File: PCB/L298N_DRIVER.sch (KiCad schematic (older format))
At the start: 21 parts, among them J1 PWM-INPUT, J2 MOT-OUTPUT, J3 +5V, J4 +BATT, J5 SERIAL, J6 I2C, U1 L298N, U2 adino2

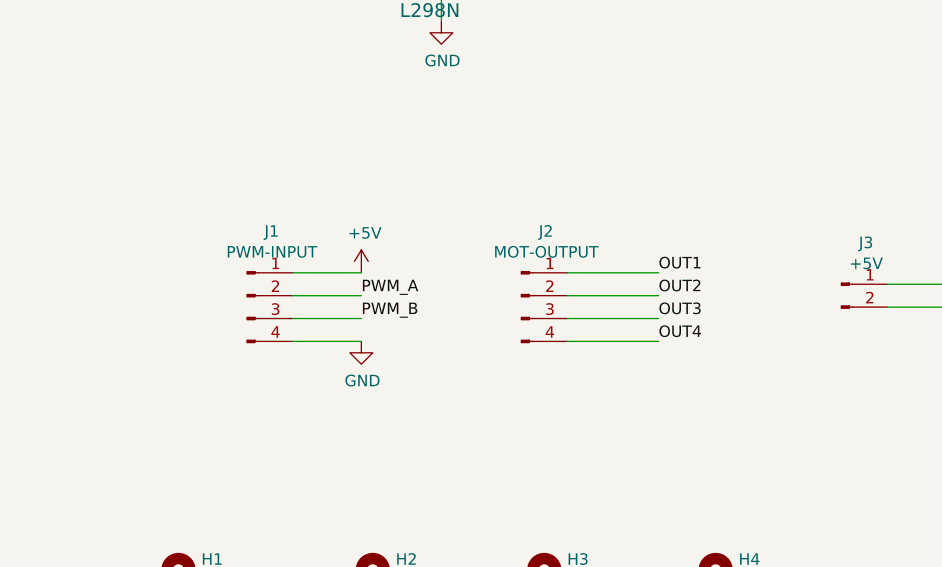
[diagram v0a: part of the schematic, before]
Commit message: pcb update
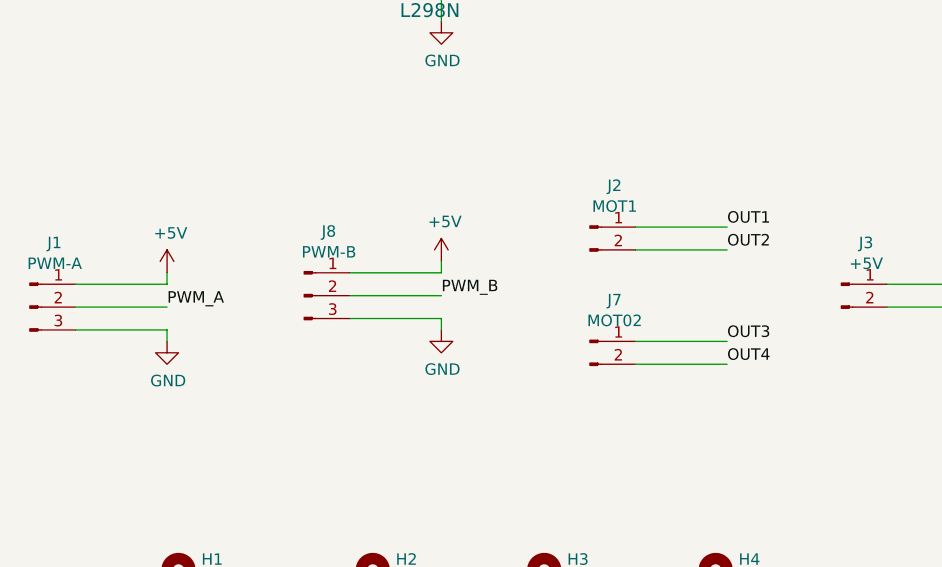
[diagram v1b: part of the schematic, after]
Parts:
- removed J1: PWM-INPUT, Connector_JST:JST_PH_S4B-PH-K_1x04_P2.00mm_Horizontal, symbol Connector:Conn_01x04_Male
- removed J2: MOT-OUTPUT, Connector_JST:JST_PH_S4B-PH-K_1x04_P2.00mm_Horizontal, symbol Connector:Conn_01x04_Male
- added J1: PWM-A, Connector_JST:JST_PH_S3B-PH-K_1x03_P2.00mm_Horizontal, symbol Connector:Conn_01x03_Male
- added J2: MOT1, Connector_JST:JST_PH_S2B-PH-K_1x02_P2.00mm_Horizontal, symbol Connector:Conn_01x02_Male
- added J7: MOT02, Connector_JST:JST_PH_S2B-PH-K_1x02_P2.00mm_Horizontal, symbol Connector:Conn_01x02_Male
- added J8: PWM-B, Connector_JST:JST_PH_S3B-PH-K_1x03_P2.00mm_Horizontal, symbol Connector:Conn_01x03_Male
- J5, J6: footprint Connector_JST:JST_PH_S4B-PH-K_1x04_P2.00mm_Horizontal -> Connector_JST:JST_PH_B4B-PH-K_1x04_P2.00mm_Vertical
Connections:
- net +5V: now also J1.1 (Pin_1), J8.1 (Pin_1)
- net GND: now also J1.3 (Pin_3), J8.3 (Pin_3)
- net OUT1: now also J2.1 (Pin_1)
- net OUT2: now also J2.2 (Pin_2)
- net OUT3: now also J7.1 (Pin_1)
- net OUT4: now also J7.2 (Pin_2)
- net PWM_A: now also J1.2 (Pin_2)
- net PWM_B: now also J8.2 (Pin_2)
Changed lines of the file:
@@
 Wire Wire Line
 	8200 3150 8600 3150
-Wire Wire Line
-	2650 5700 2950 5700
 $Comp
 L power:GND #PWR04
 U 1 1 5E721439
-P 2950 5700
-F 0 "#PWR04" H 2950 5450 50  0001 C CNN
-F 1 "GND" H 2955 5527 50  0000 C CNN
-F 2 "" H 2950 5700 50  0001 C CNN
-F 3 "" H 2950 5700 50  0001 C CNN
-	1    2950 5700
+P 2100 5700
+F 0 "#PWR04" H 2100 5450 50  0001 C CNN
+F 1 "GND" H 2105 5527 50  0000 C CNN
+F 2 "" H 2100 5700 50  0001 C CNN
+F 3 "" H 2100 5700 50  0001 C CNN
+	1    2100 5700
 	1    0    0    -1
 $EndComp
@@
 Text Label 8600 3150 0    50   ~ 0
 PWM_B
-Text Label 2950 5500 0    50   ~ 0
+Text Label 2100 5550 0    50   ~ 0
 PWM_A
-Text Label 2950 5600 0    50   ~ 0
-PWM_B
 $Comp
 L power:GND #PWR013
@@
 $EndComp
 $Comp
-L Connector:Conn_01x04_Male J1
-U 1 1 5E80A4BE
-P 2450 5500
-F 0 "J1" H 2558 5781 50  0000 C CNN
-F 1 "PWM-INPUT" H 2558 5690 50  0000 C CNN
-F 2 "Connector_JST:JST_PH_S4B-PH-K_1x04_P2.00mm_Horizontal" H 2450 5500 50  0001 C CNN
-F 3 "~" H 2450 5500 50  0001 C CNN
-	1    2450 5500
-	1    0    0    -1
-$EndComp
-Wire Wire Line
-	2650 5500 2950 5500
-Wire Wire Line
-	2650 5600 2950 5600
-$Comp
 L power:+5V #PWR06
 U 1 1 5E80EB83
-P 2950 5400
-F 0 "#PWR06" H 2950 5250 50  0001 C CNN
-F 1 "+5V" H 2965 5573 50  0000 C CNN
-F 2 "" H 2950 5400 50  0001 C CNN
-F 3 "" H 2950 5400 50  0001 C CNN
-	1    2950 5400
-	1    0    0    -1
-$EndComp
-$Comp
-L Connector:Conn_01x04_Male J2
-U 1 1 5E81BECC
-P 3650 5500
-F 0 "J2" H 3758 5781 50  0000 C CNN
-F 1 "MOT-OUTPUT" H 3758 5690 50  0000 C CNN
-F 2 "Connector_JST:JST_PH_S4B-PH-K_1x04_P2.00mm_Horizontal" H 3650 5500 50  0001 C CNN
-F 3 "~" H 3650 5500 50  0001 C CNN
-	1    3650 5500
-	1    0    0    -1
-$EndComp
-Text Label 4250 5400 0    50   ~ 0
+P 2100 5400
+F 0 "#PWR06" H 2100 5250 50  0001 C CNN
+F 1 "+5V" H 2115 5573 50  0000 C CNN
+F 2 "" H 2100 5400 50  0001 C CNN
+F 3 "" H 2100 5400 50  0001 C CNN
+	1    2100 5400
+	1    0    0    -1
+$EndComp
+Text Label 4550 5200 0    50   ~ 0
 OUT1
-Text Label 4250 5500 0    50   ~ 0
+Text Label 4550 5300 0    50   ~ 0
 OUT2
 Wire Wire Line
-	3850 5700 4250 5700
-Text Label 4250 5700 0    50   ~ 0
+	4150 5800 4550 5800
+Text Label 4550 5800 0    50   ~ 0
 OUT4
-Text Label 4250 5600 0    50   ~ 0
+Text Label 4550 5700 0    50   ~ 0
 OUT3
 Wire Wire Line
-	3850 5600 4250 5600
-Wire Wire Line
-	3850 5400 4250 5400
-Wire Wire Line
-	3850 5500 4250 5500
+	4150 5700 4550 5700
+Wire Wire Line
+	4150 5200 4550 5200
+Wire Wire Line
+	4150 5300 4550 5300
 $Comp
 L Connector:Conn_01x04_Male J5
@@
 F 0 "J5" H 7508 5731 50  0000 C CNN
 F 1 "SERIAL" H 7508 5640 50  0000 C CNN
-F 2 "Connector_JST:JST_PH_S4B-PH-K_1x04_P2.00mm_Horizontal" H 7400 5450 50  0001 C CNN
+F 2 "Connector_JST:JST_PH_B4B-PH-K_1x04_P2.00mm_Vertical" H 7400 5450 50  0001 C CNN
 F 3 "~" H 7400 5450 50  0001 C CNN
 	1    7400 5450
@@
 F 0 "J6" H 8908 5731 50  0000 C CNN
 F 1 "I2C" H 8908 5640 50  0000 C CNN
-F 2 "Connector_JST:JST_PH_S4B-PH-K_1x04_P2.00mm_Horizontal" H 8800 5450 50  0001 C CNN
+F 2 "Connector_JST:JST_PH_B4B-PH-K_1x04_P2.00mm_Vertical" H 8800 5450 50  0001 C CNN
 F 3 "~" H 8800 5450 50  0001 C CNN
 	1    8800 5450
@@
 Text Label 9650 5550 0    50   ~ 0
 SDA
-Wire Wire Line
-	2650 5400 2950 5400
+$Comp
+L Connector:Conn_01x02_Male J2
+U 1 1 5E811B91
+P 3950 5200
+F 0 "J2" H 4058 5381 50  0000 C CNN
+F 1 "MOT1" H 4058 5290 50  0000 C CNN
+F 2 "Connector_JST:JST_PH_S2B-PH-K_1x02_P2.00mm_Horizontal" H 3950 5200 50  0001 C CNN
+F 3 "~" H 3950 5200 50  0001 C CNN
+	1    3950 5200
+	1    0    0    -1
+$EndComp
+$Comp
+L Connector:Conn_01x02_Male J7
+U 1 1 5E8159E2
+P 3950 5700
+F 0 "J7" H 4058 5881 50  0000 C CNN
+F 1 "MOT02" H 4058 5790 50  0000 C CNN
+F 2 "Connector_JST:JST_PH_S2B-PH-K_1x02_P2.00mm_Horizontal" H 3950 5700 50  0001 C CNN
+F 3 "~" H 3950 5700 50  0001 C CNN
+	1    3950 5700
+	1    0    0    -1
+$EndComp
+$Comp
+L Connector:Conn_01x03_Male J1
+U 1 1 5E8405FC
+P 1500 5550
+F 0 "J1" H 1608 5831 50  0000 C CNN
+F 1 "PWM-A" H 1608 5740 50  0000 C CNN
+F 2 "Connector_JST:JST_PH_S3B-PH-K_1x03_P2.00mm_Horizontal" H 1500 5550 50  0001 C CNN
+F 3 "~" H 1500 5550 50  0001 C CNN
+	1    1500 5550
+	1    0    0    -1
+$EndComp
+$Comp
+L power:GND #PWR020
+U 1 1 5E84B54A
+P 3300 5650
+F 0 "#PWR020" H 3300 5400 50  0001 C CNN
+F 1 "GND" H 3305 5477 50  0000 C CNN
+F 2 "" H 3300 5650 50  0001 C CNN
+F 3 "" H 3300 5650 50  0001 C CNN
+	1    3300 5650
+	1    0    0    -1
+$EndComp
+$Comp
+L power:+5V #PWR019
+U 1 1 5E84B551
+P 3300 5350
+F 0 "#PWR019" H 3300 5200 50  0001 C CNN
+F 1 "+5V" H 3315 5523 50  0000 C CNN
+F 2 "" H 3300 5350 50  0001 C CNN
+F 3 "" H 3300 5350 50  0001 C CNN
+	1    3300 5350
+	1    0    0    -1
+$EndComp
+Wire Wire Line
+	1700 5450 2100 5450
+Wire Wire Line
+	2100 5450 2100 5400
+Wire Wire Line
+	1700 5550 2100 5550
+Wire Wire Line
+	1700 5650 2100 5650
+Wire Wire Line
+	2100 5650 2100 5700
+Wire Wire Line
+	3300 5400 3300 5350
+Text Label 3300 5500 0    50   ~ 0
+PWM_B
+$Comp
+L Connector:Conn_01x03_Male J8
+U 1 1 5E84B557
+P 2700 5500
+F 0 "J8" H 2808 5781 50  0000 C CNN
+F 1 "PWM-B" H 2808 5690 50  0000 C CNN
+F 2 "Connector_JST:JST_PH_S3B-PH-K_1x03_P2.00mm_Horizontal" H 2700 5500 50  0001 C CNN
+F 3 "~" H 2700 5500 50  0001 C CNN
+	1    2700 5500
+	1    0    0    -1
+$EndComp
+Wire Wire Line
+	2900 5500 3300 5500
+Wire Wire Line
+	2900 5600 3300 5600
+Wire Wire Line
+	3300 5600 3300 5650
+Wire Wire Line
+	2900 5400 3300 5400
 $EndSCHEMATC
